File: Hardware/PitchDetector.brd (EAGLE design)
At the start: 81.3 x 93.2 mm, 46 parts, among them IC1 STM32F302CBT6, IC2 LM3940IMP-3.3_NOPB, X1 MINI-USB-32005-201, X2 HD44780LCD-1602, Y1 ABLS-8.000MHZ-K4T

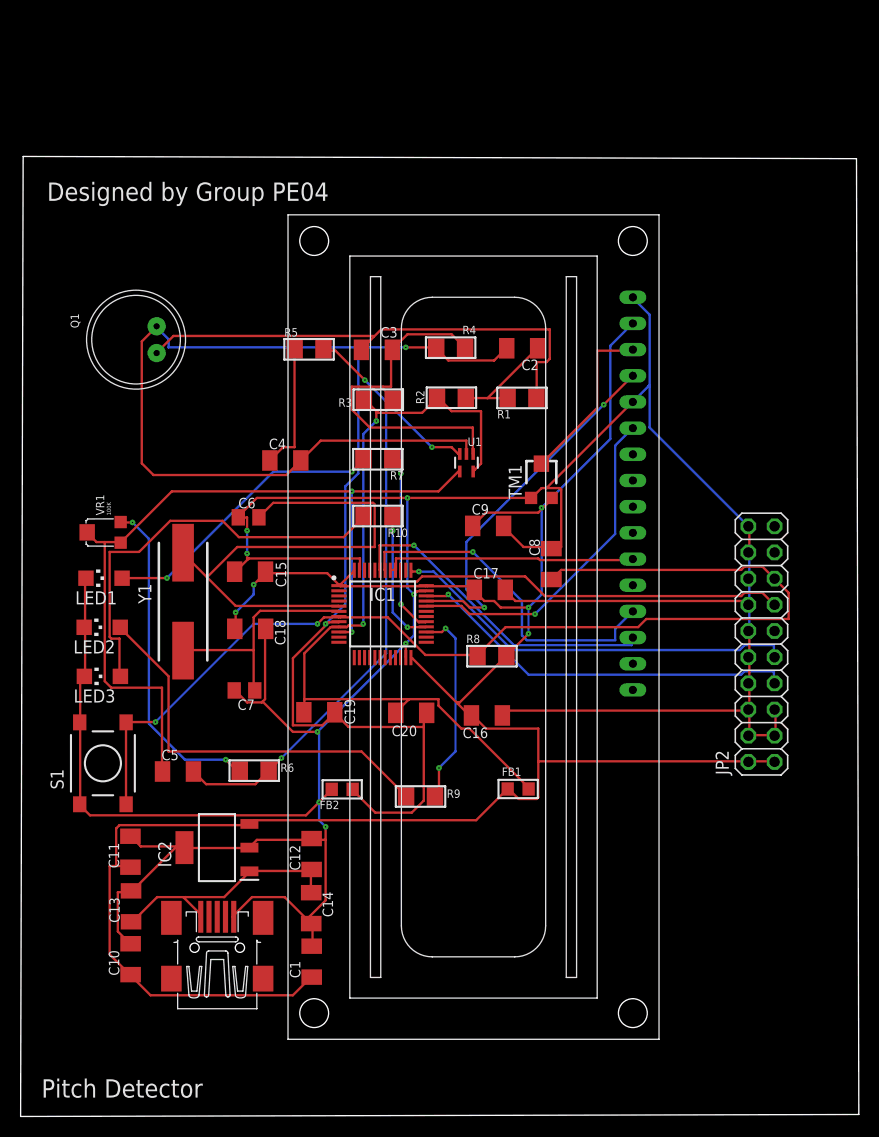
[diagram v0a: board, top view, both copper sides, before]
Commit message: PCB updated.
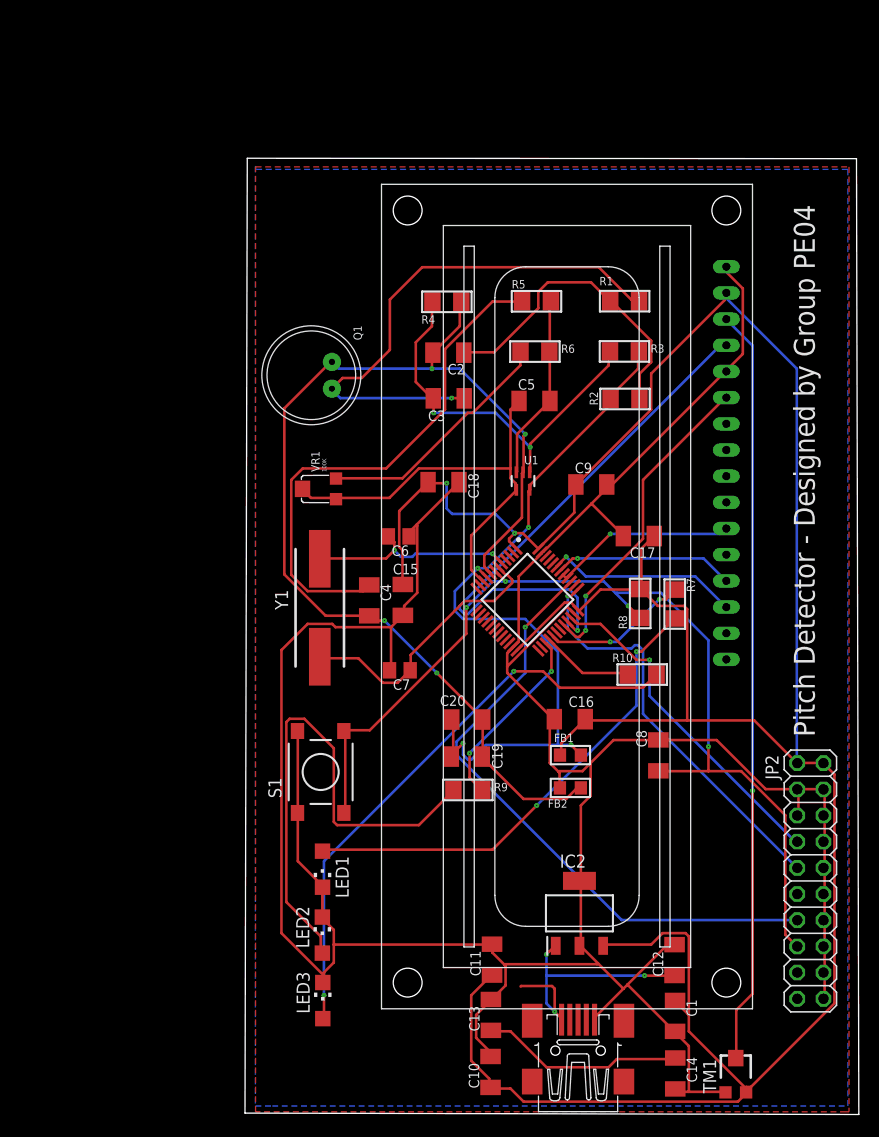
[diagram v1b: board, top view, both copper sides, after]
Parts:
- moved TM1 60.7 mm to (111.4, 5.10)
- moved C5 49.9 mm to (91.9, 70.4)
- moved R6 48.9 mm to (91.9, 75.2)
- moved C14 38.8 mm to (105.5, 5.11)
- moved LED3 38.0 mm to (71.3, 12.2), turned to 0 degrees
- moved LED2 36.7 mm to (71.3, 18.5), turned to 0 degrees
- moved C12 36.7 mm to (105.5, 16.1)
- moved C11 36.6 mm to (87.7, 16.2)
- moved C10 36.6 mm to (87.6, 5.26)
- moved C13 36.5 mm to (87.6, 10.8)
- moved X1 36.4 mm to (96.1, 7.33)
- moved IC2 35.7 mm to (96.2, 20.6), turned to 90 degrees
- moved C1 35.7 mm to (105.5, 10.7), turned to 270 degrees
- moved LED1 35.3 mm to (71.3, 24.9), turned to 180 degrees
- moved R7 32.0 mm to (105.5, 50.7), turned to 90 degrees
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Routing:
- net 3V3: track 213.2 -> 278.6 mm, vias 5 -> 2
- net N$10: track 16.7 -> 73.4 mm, vias 0 -> 1
- net CGND: track 156.6 -> 108.0 mm, vias 2 -> 4
- net IN-: track 66.3 -> 18.1 mm, vias 3 -> 0
- net ADC0: track 81.8 -> 42.4 mm, vias 2 -> 0
- net N$9: track 12.4 -> 50.7 mm
- net XTAL1: track 50.8 -> 20.6 mm, vias 0 -> 2
- net GND: track 339.7 -> 317.1 mm, vias 8 -> 0
- net SWO: track 38.9 -> 61.2 mm, vias 0 -> 1
- net VUSB: track 24.4 -> 46.1 mm, vias 0 -> 3
- net N$6: track 10.9 -> 30.5 mm
- net N$1: track 28.2 -> 46.6 mm
- net LCD_RS: track 35.8 -> 54.1 mm, vias 2 -> 1
- net N$11: track 40.5 -> 56.5 mm, vias 0 -> 2
- net LCD_D6: track 33.2 -> 17.5 mm
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- added copper zone on layer 1, net GND
- added copper zone on layer 16, net GND
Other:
- board size 81.3 x 93.2 mm -> 59.6 x 92.8 mm
- board text added: "Pitch Detector - Designed by Group PE04"
- board text removed: "Designed by Group PE04"
- board text removed: "Pitch Detector"
